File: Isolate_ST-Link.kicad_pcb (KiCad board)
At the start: 2 copper layers, 39 x 38 mm, 70 parts, among them J1 USB_OTG, J2 CONN_01X06, J3 CONN_01X04, J4 CONN_01X02, J5 CONN_01X02, J6 GS2, Q1 BSS138, U1 MAU10x, U2 ADuM4160, U3 APE8865NR-33-HF-3, U4 STM32F103CBTx, Y1 Crystal

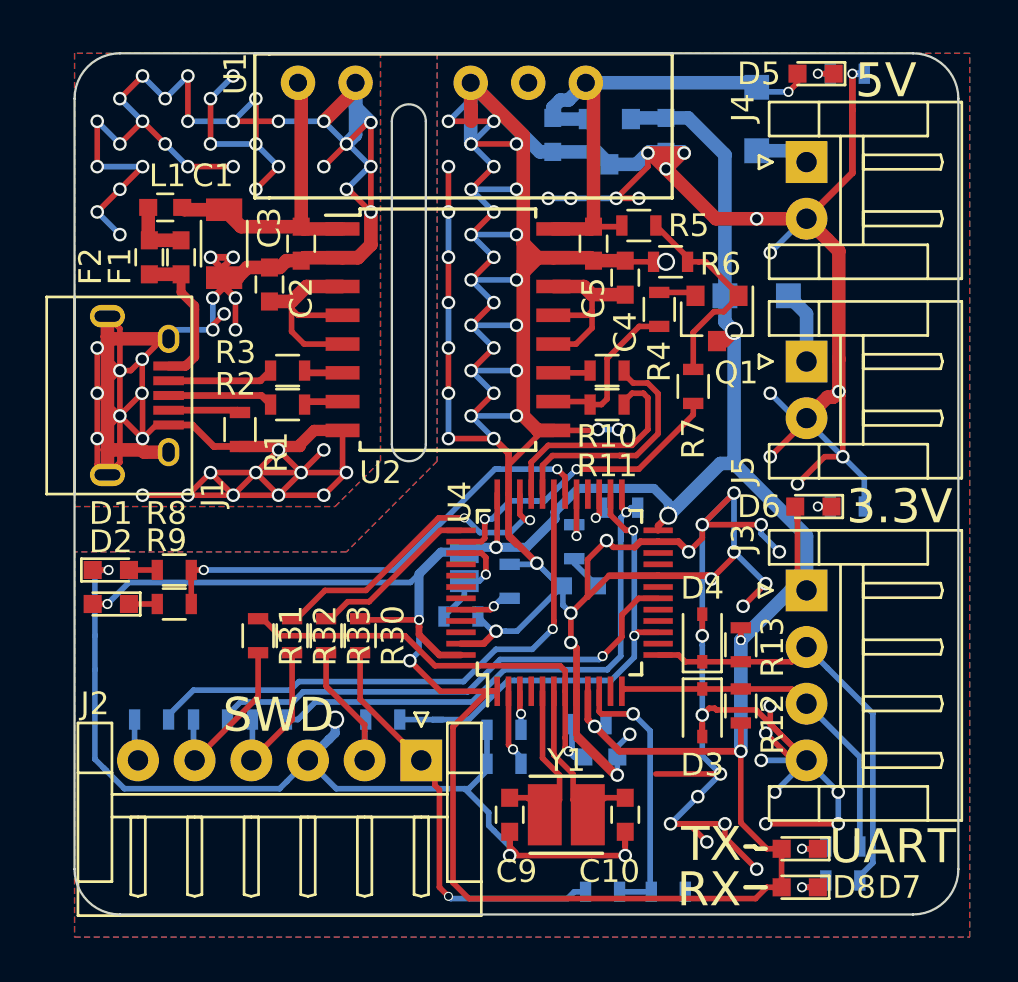
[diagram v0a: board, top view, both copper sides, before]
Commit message: 進捗
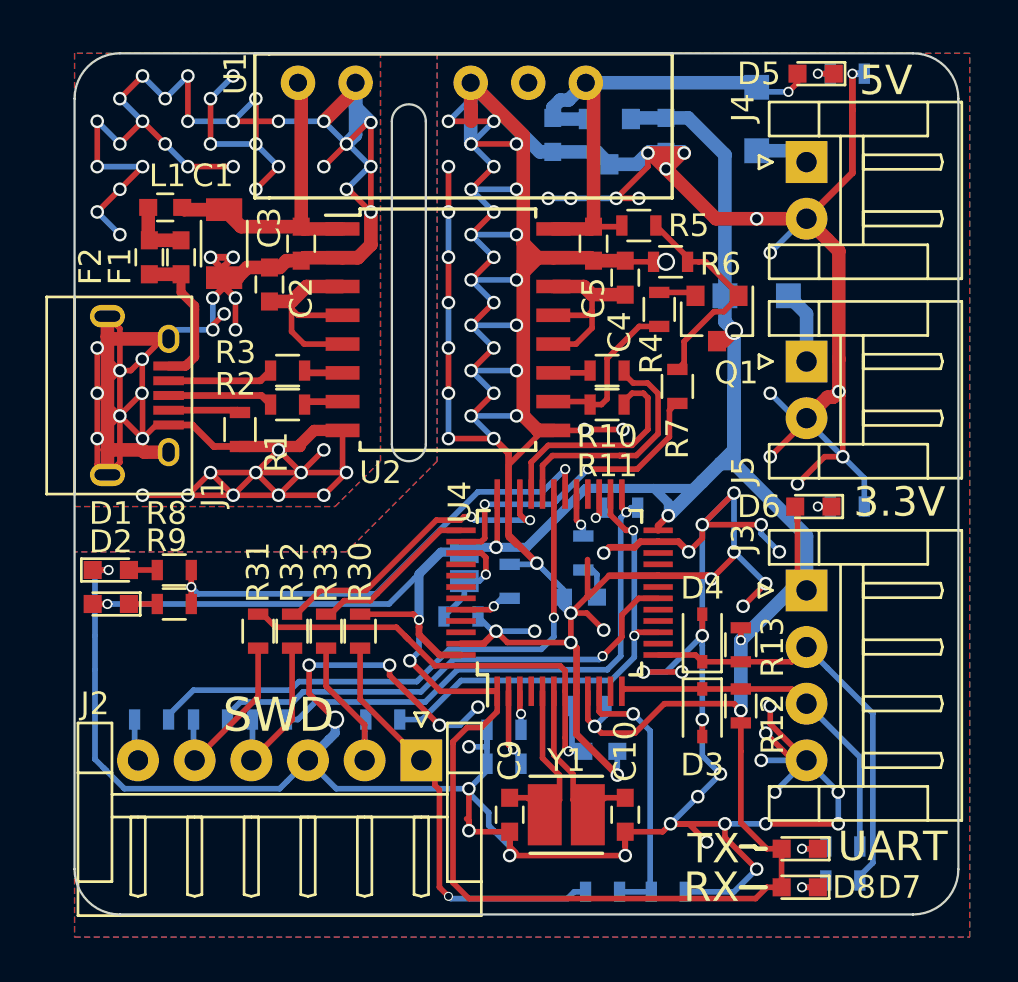
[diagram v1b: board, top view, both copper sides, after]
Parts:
- moved R21 0.80 mm to (176.2, 78.8)
- moved R7 0.70 mm to (180.1, 64.7)
- moved R26 0.64 mm to (175.9, 72.0)
- moved C11 0.50 mm to (175.8, 74.0)
- moved C8 0.25 mm to (176.7, 80.8)
- moved R30 0.20 mm to (166.1, 75.5)
- moved R31 0.20 mm to (161.6, 75.5)
- moved R32 0.20 mm to (163.1, 75.5)
- moved R33 0.20 mm to (164.6, 75.5)
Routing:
- net GND: track 318.4 -> 336.2 mm, vias 83 -> 93
- net SYS_NRST: track 20.1 -> 21.1 mm
- net T_JTMS: track 24.8 -> 23.9 mm
- net +3V3: track 137.5 -> 138.4 mm
- net /MCU/LED_STLINK: track 20.9 -> 21.5 mm
